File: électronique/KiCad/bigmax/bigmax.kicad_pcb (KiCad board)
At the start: 2 copper layers, 190.5 x 94 mm, 31 parts, among them J1 Conn_01x03, J2 Conn_01x02, J3 Conn_01x03_input, J4 Conn_01x02, SW1 SW_Push, U1 pololu_enc03b, U10 jsumo_micro_start, U11 generic_vertical_slide_switch, U12 generic_bms_3s_10A, U13 generic_18650_3s_case, U2 pololu_enc03b, U3 pololu_irs01a, U4 pololu_irs01a, U5 pololu_reg19a, U6 pololu_reg04b, U7 pololu_md17a, U8 generic_vl53l0x, U9 generic_vl53l0x

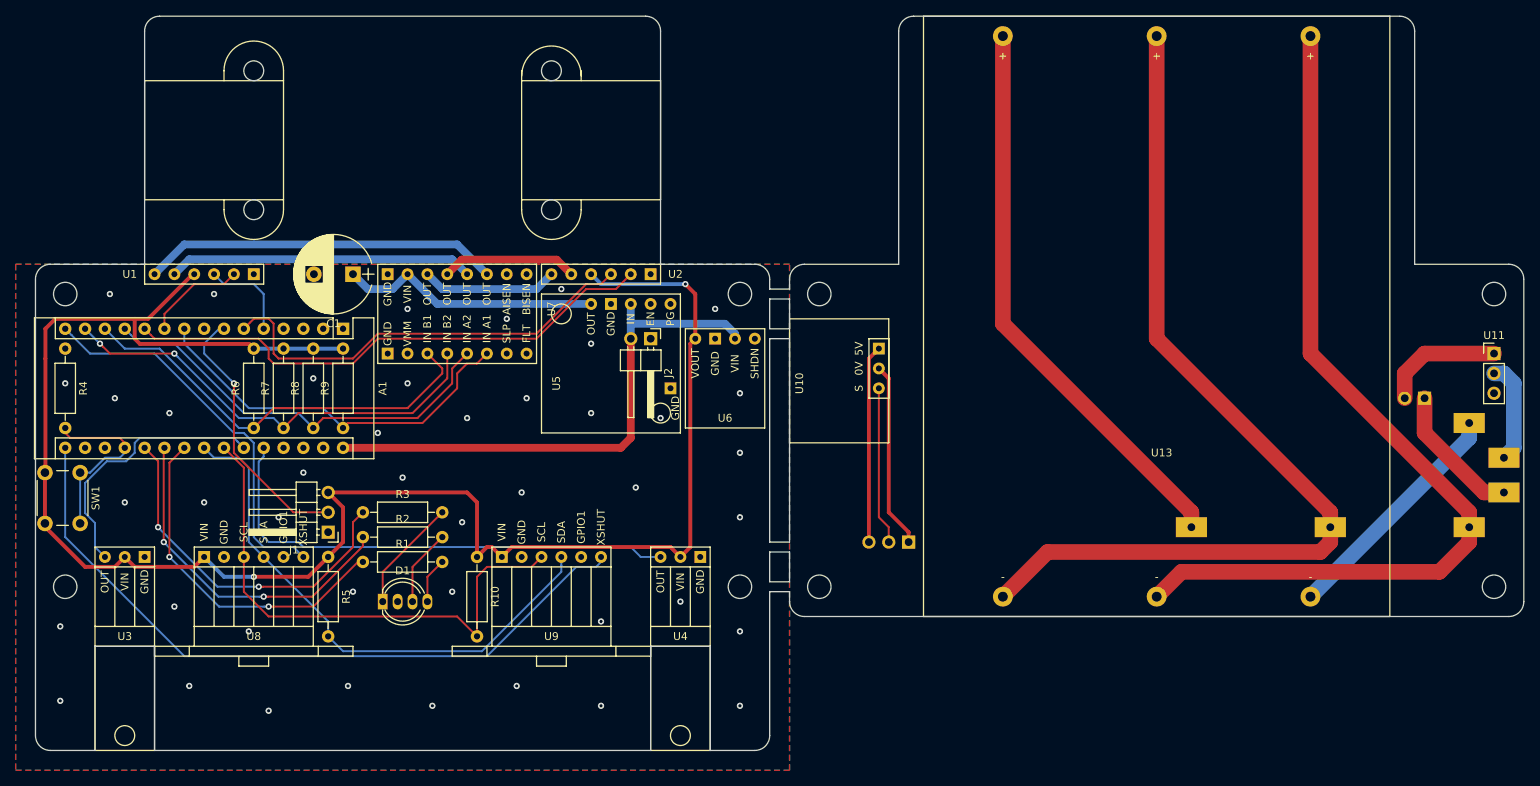
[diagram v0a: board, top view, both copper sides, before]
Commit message: first 22 push
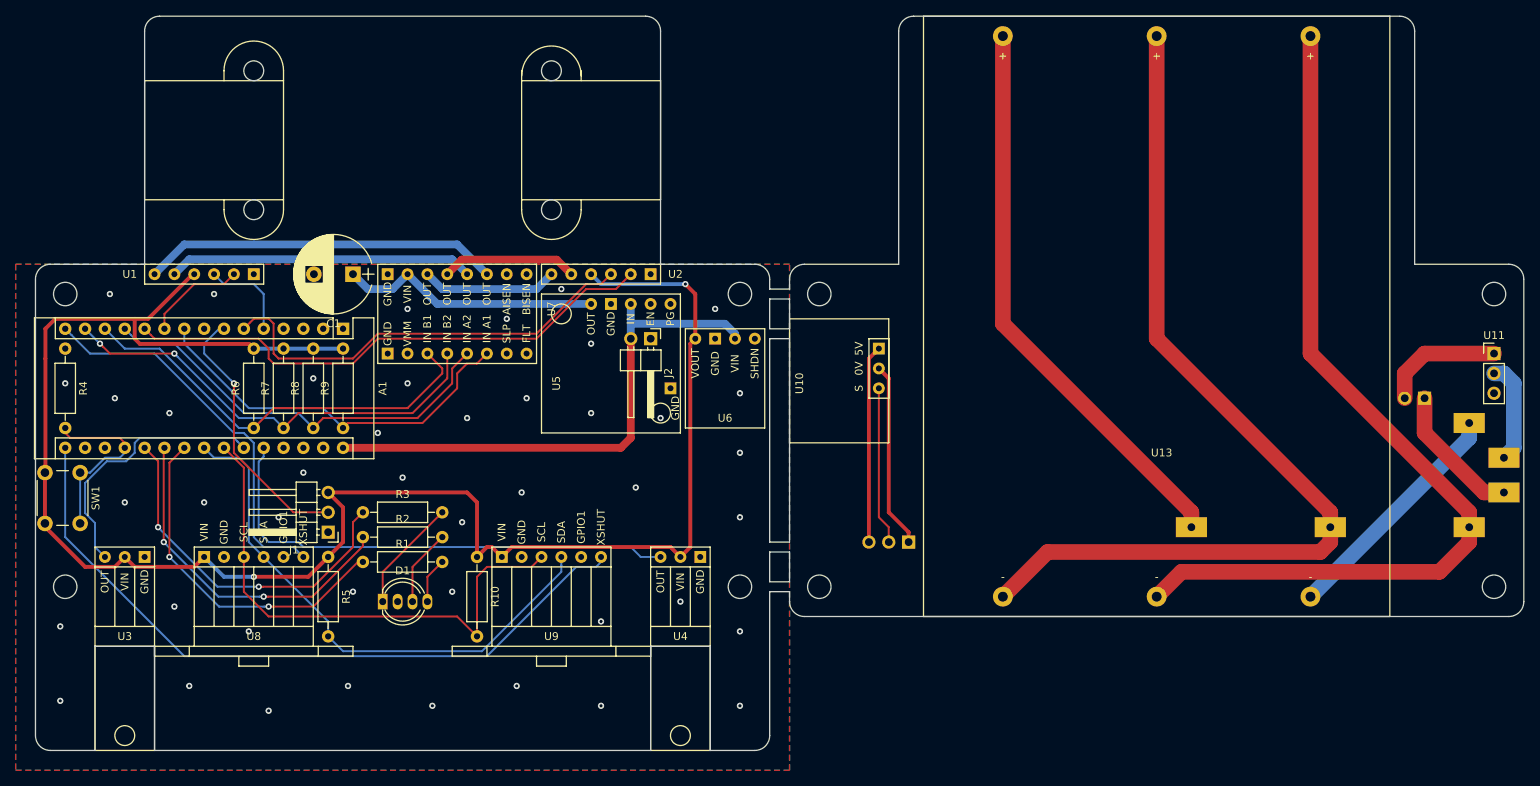
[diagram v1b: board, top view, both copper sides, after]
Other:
- net class Default removed
